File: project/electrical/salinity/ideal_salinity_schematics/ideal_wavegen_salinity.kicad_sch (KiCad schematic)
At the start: 12 parts, among them U2 MCP6001-OT, U3 MCP6001-OT, U3 U1, U4 MCP6001-OT

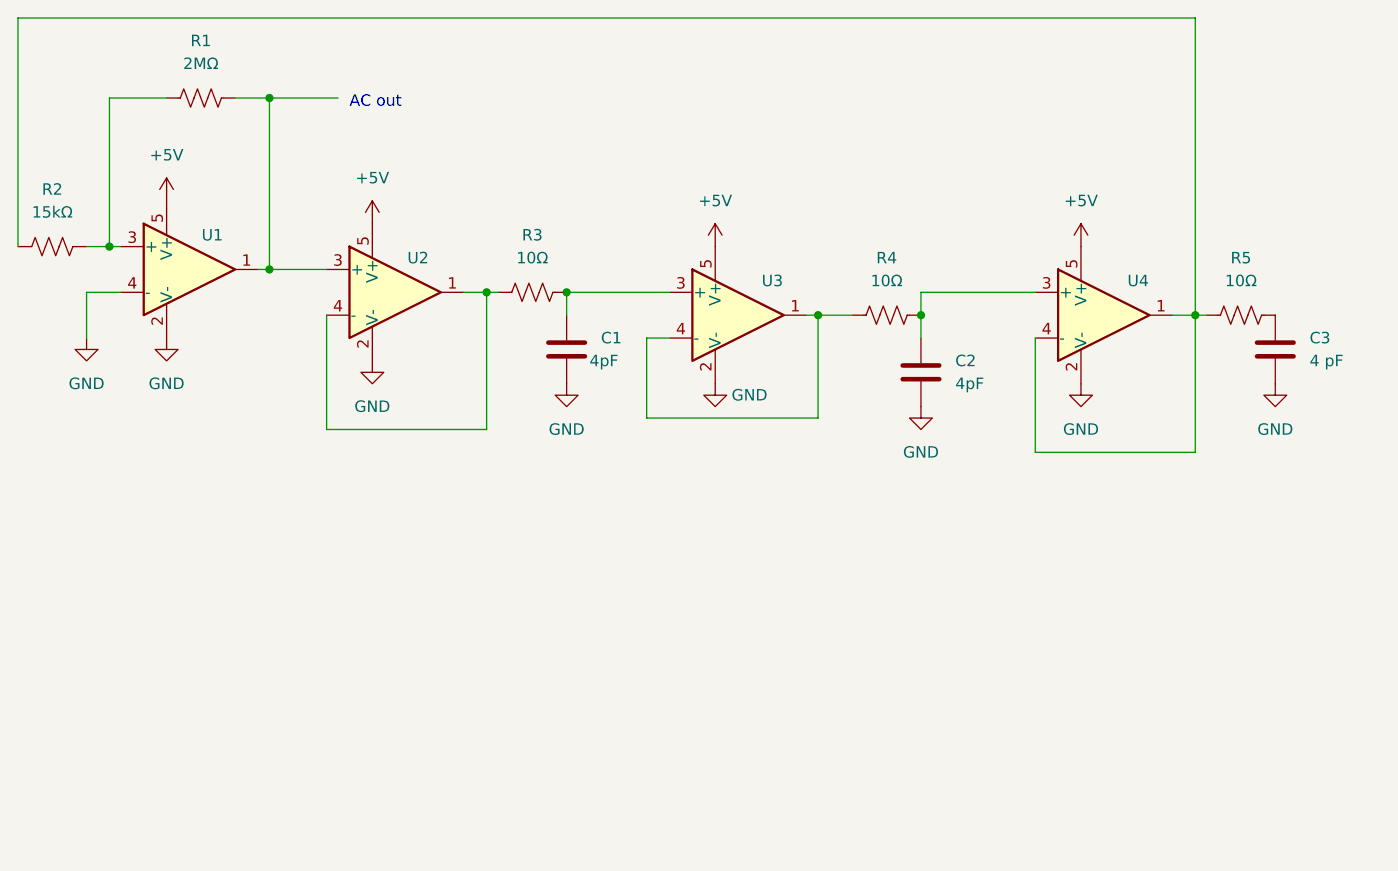
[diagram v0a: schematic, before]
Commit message: Made some circuits better for overleaf
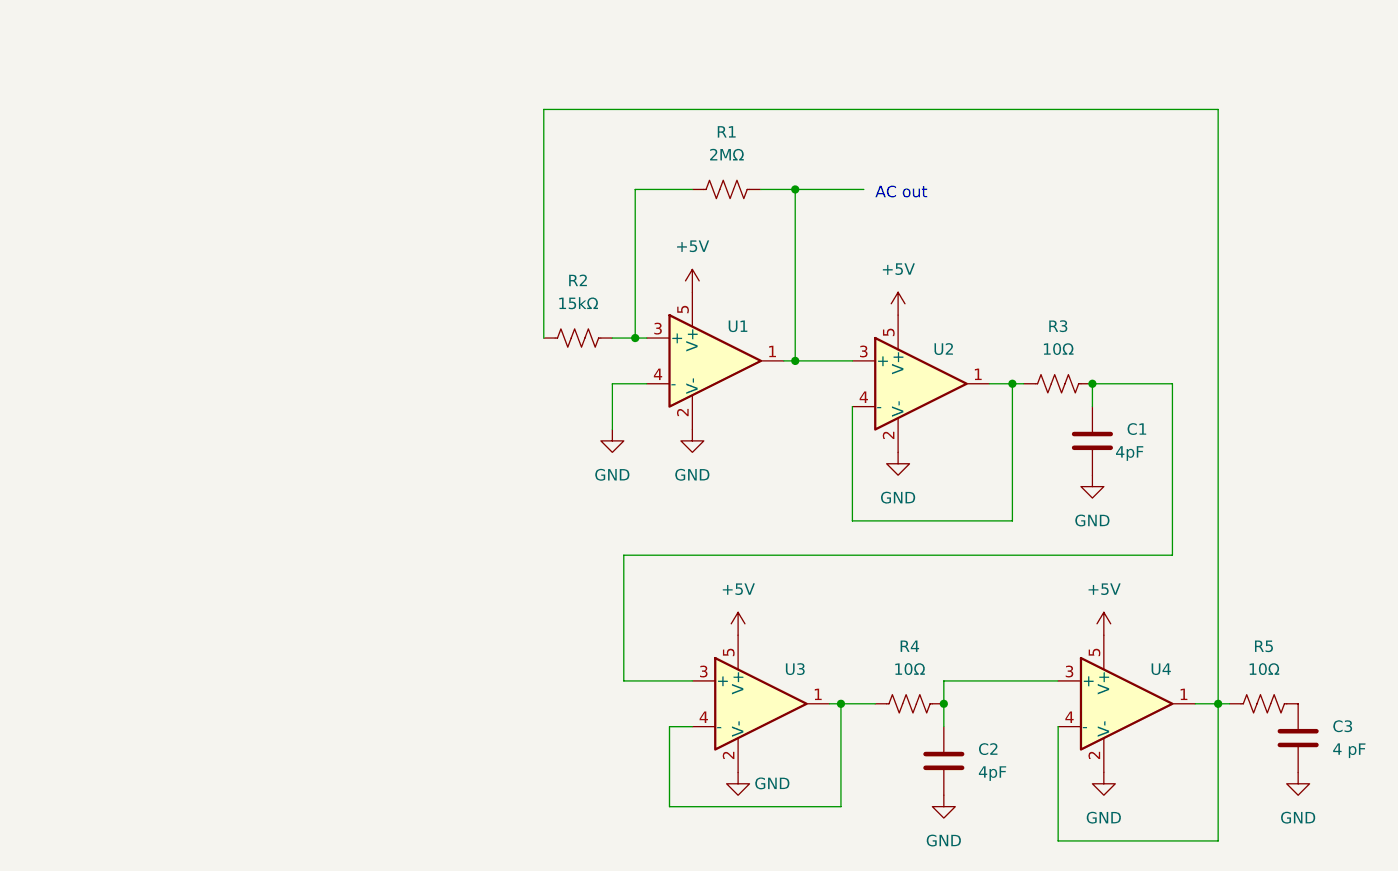
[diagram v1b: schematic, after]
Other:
- moved on the sheet: C1, C2, C3, R1, R2, R3, R4, R5, U2, U3, U4
